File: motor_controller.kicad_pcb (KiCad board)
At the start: 4 copper layers, 43.7 x 46.5 mm, 36 parts, among them IC1 DRV8304SRHAR, J1 PWM, J2 SPI, J3 MISC, J4 PWR IN, J5 MOTOR, Q1 CSD18514Q5A, Q2 CSD18514Q5A, Q3 CSD18514Q5A, Q4 CSD18514Q5A, Q5 CSD18514Q5A, Q6 CSD18514Q5A

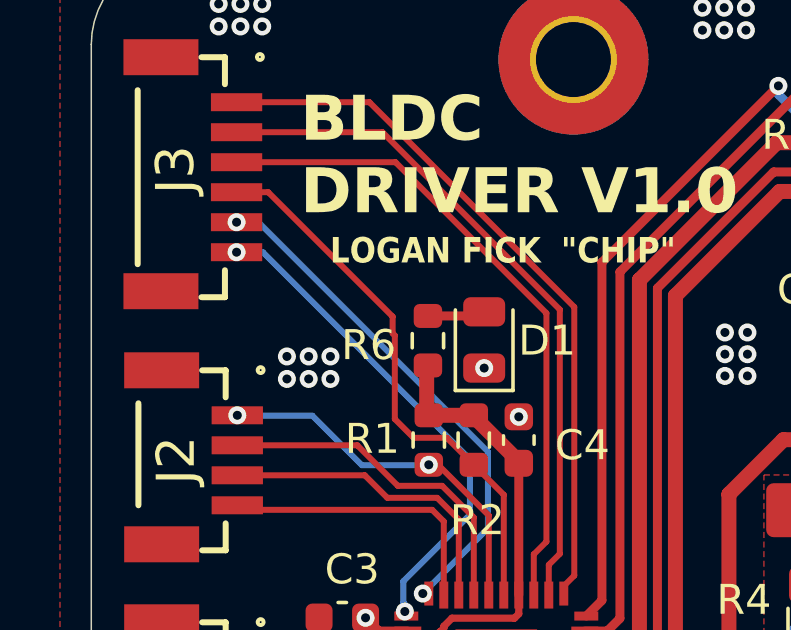
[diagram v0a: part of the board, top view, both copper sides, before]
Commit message: revision 1.0 ordered
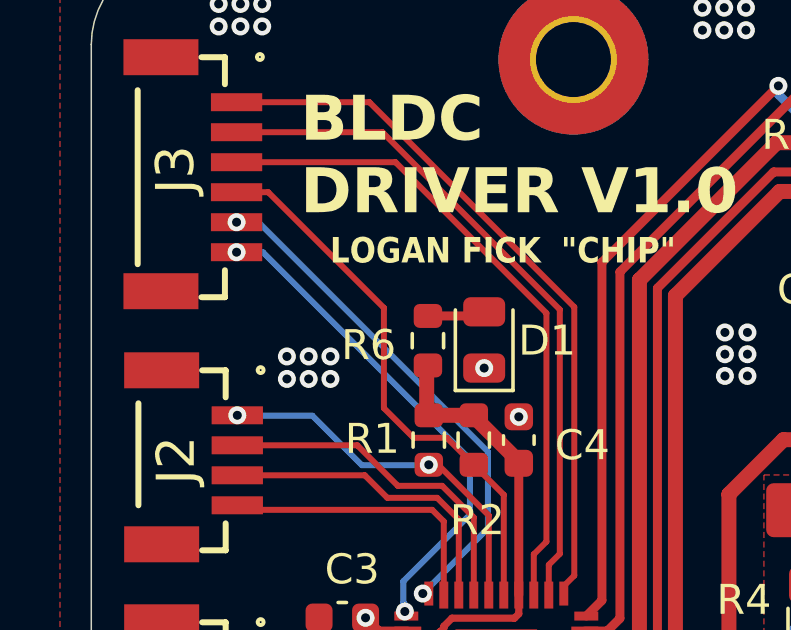
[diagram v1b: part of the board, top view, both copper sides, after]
